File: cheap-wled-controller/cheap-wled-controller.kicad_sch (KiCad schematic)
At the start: 6 parts, among them CN1 WJ124-3.81-5P-14-00A, U1 AMS1117-3.3, U2 ESP32-S3-WROOM-1-N4R2, U3 ZX-PZ2.0-2-5PZZ, U4 74LV1T34GWH_C5199768

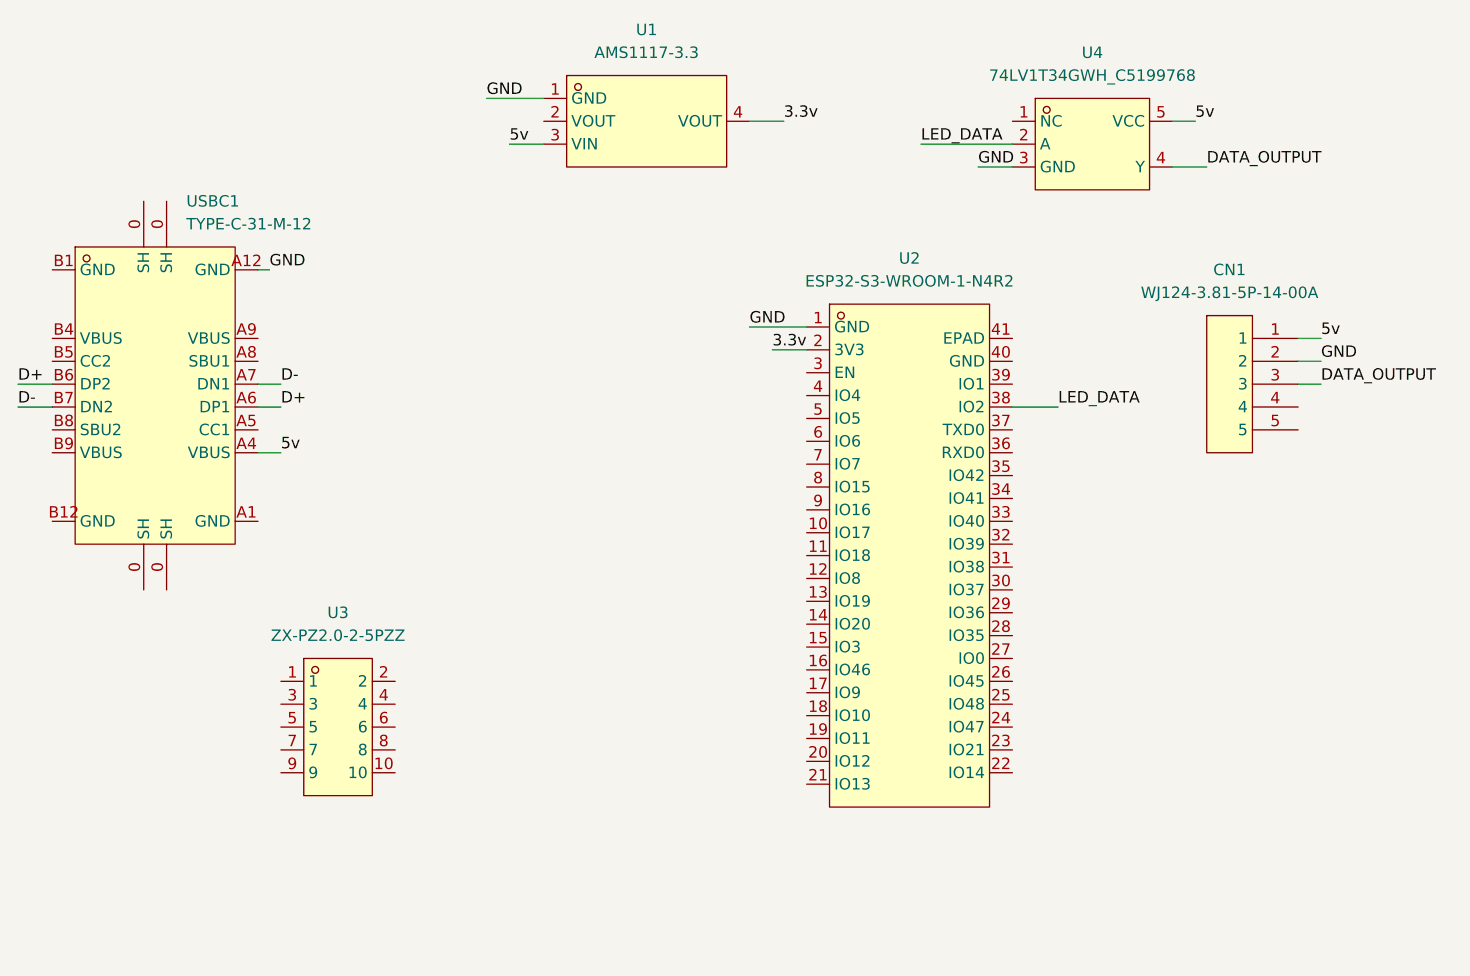
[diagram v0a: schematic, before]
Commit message: voltage selector
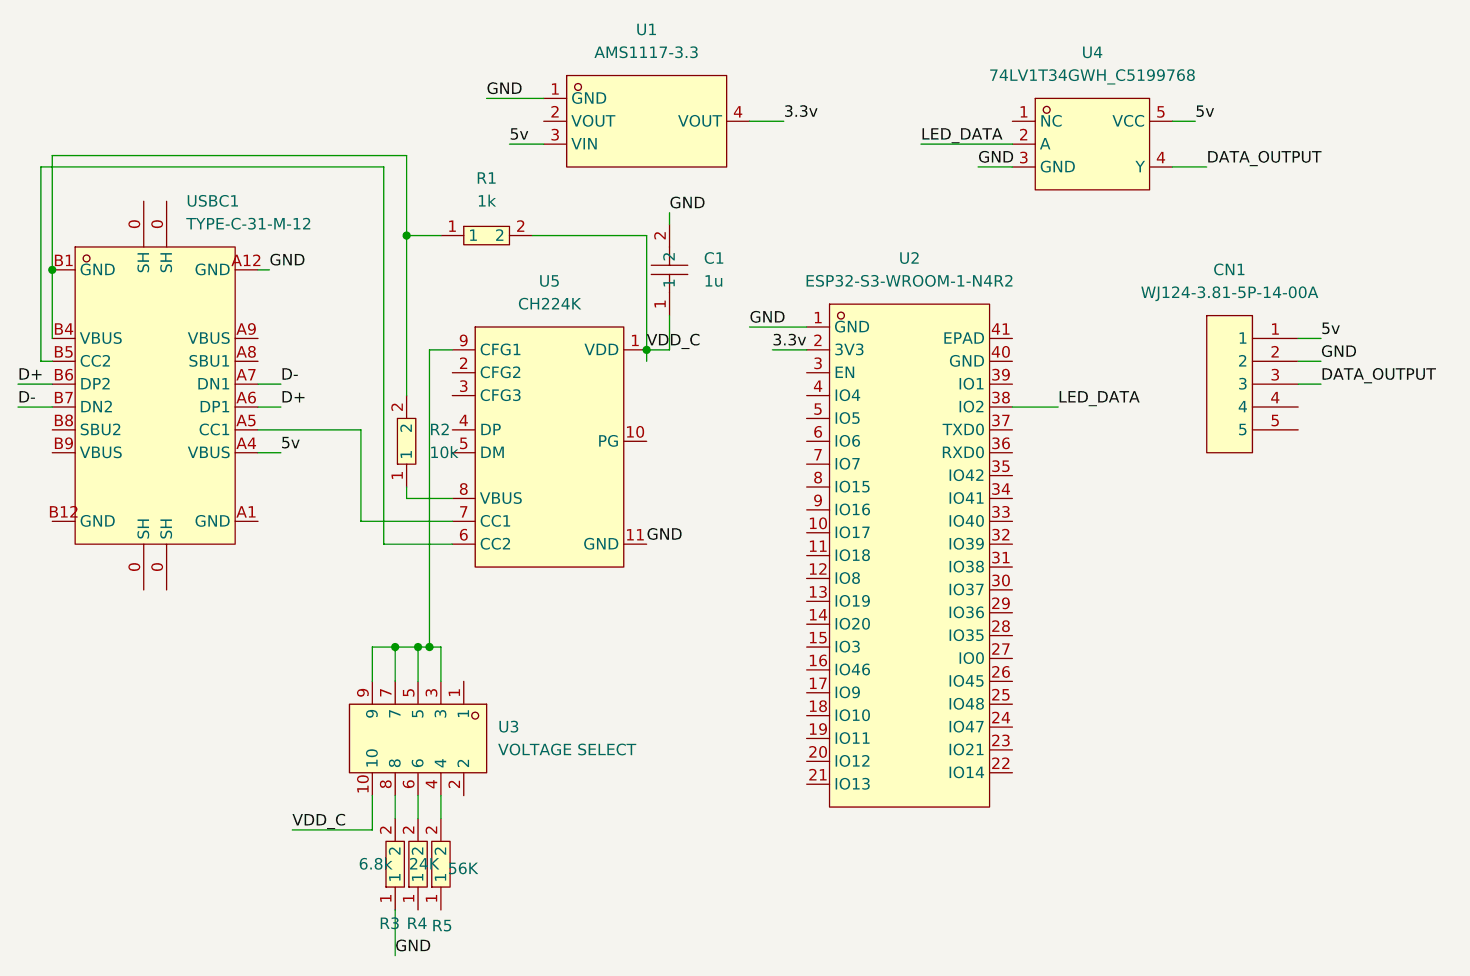
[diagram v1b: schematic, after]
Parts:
- added C1: 1u, cheap-wled-controller:C0805, symbol easyeda:0805B105K500NT_C215803
- added R1: 1k, cheap-wled-controller:R0805, symbol easyeda:0805W8F1001T5E
- added R2: 10k, cheap-wled-controller:R0805, symbol easyeda:0805W8F1002T5E
- added R3: 6.8k, cheap-wled-controller:R0805, symbol easyeda:0805W8F6801T5E
- added R4: 24K, cheap-wled-controller:R0805, symbol easyeda:0805W8F2402T5E
- added R5: 56K, cheap-wled-controller:R0805, symbol easyeda:0805W8F5602T5E
- added U5: CH224K, cheap-wled-controller:ESSOP-10_L4.9-W3.9-P1.0-LS6.0-TL-EP, symbol easyeda:CH224K
- U3: value ZX-PZ2.0-2-5PZZ -> VOLTAGE SELECT
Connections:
- net GND: now also C1.2, R3.1, U5.11 (GND)
- net at USBC1.A5 (CC1): now also U5.7 (CC1)
- net at USBC1.B1 (GND): now also USBC1.B4 (VBUS), R1.1, R2.2
- net at USBC1.B5 (CC2): now also U5.6 (CC2)
- net VDD_C: now reaches U3.10
- net VDD_C: now also C1.1, R1.2, U5.1 (VDD)
- net at U3.3: now also U3.5, U3.7, U3.9, U5.9 (CFG1)
- net at U3.4: now also R5.2
- net at U3.6: now also R4.2
- net at U3.8: now also R3.2
- new net: R2.1, U5.8 (VBUS)
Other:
- moved on the sheet: U3
